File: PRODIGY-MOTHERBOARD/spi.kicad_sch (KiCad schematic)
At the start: 3 parts, among them U13 TXS0108EPW

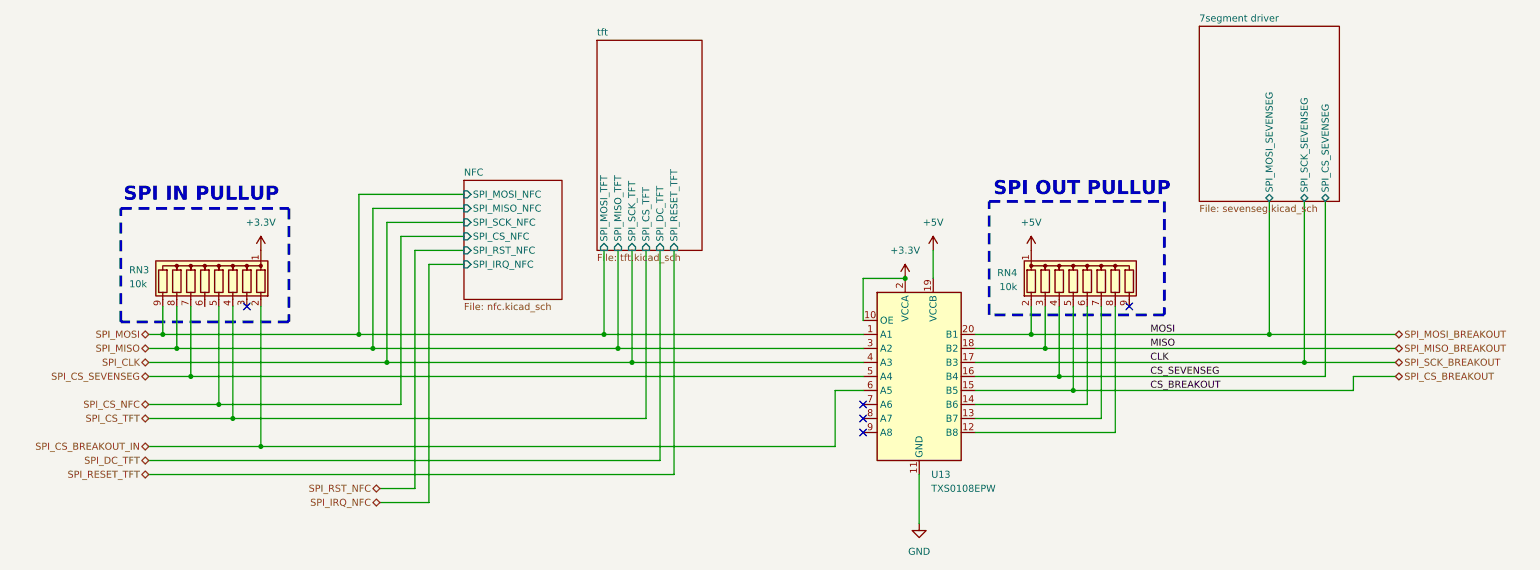
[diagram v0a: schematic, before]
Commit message: schematic v0.2 finalized
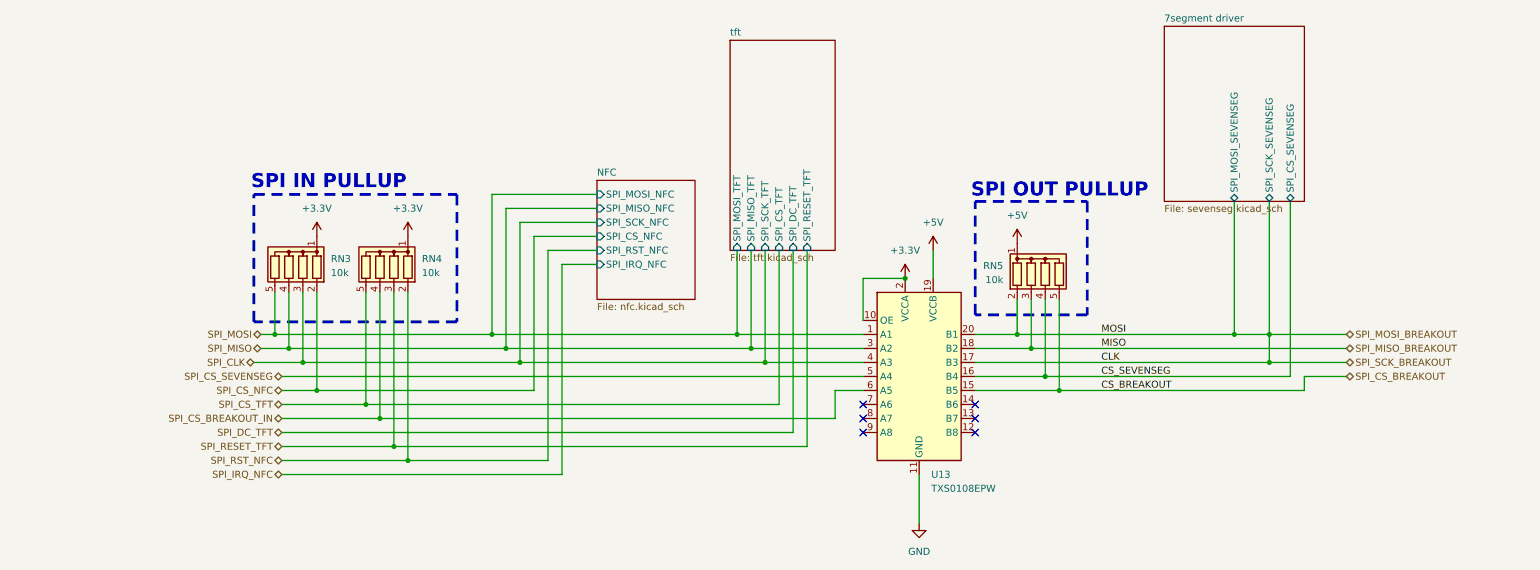
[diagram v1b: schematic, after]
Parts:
- removed RN3, RN4: 10k, Resistor_SMD:R_Array_Convex_5x0603, symbol Device:R_Network08
- added RN3, RN4, RN5: 10k, Resistor_SMD:R_Array_Convex_4x0603, symbol Device:R_Network04
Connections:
- net SPI_SCK_BREAKOUT is gone; now on net SPI_MOSI_BREAKOUT: U13.17 (B3)
- net +3.3V: now also RN3.1 (common), RN4.1 (common)
- net +5V: now also RN5.1 (common)
- net CS_SEVENSEG: now also RN5.4 (R3)
- net SPI_CLK: now also RN3.3 (R2)
- net SPI_CS_BREAKOUT: now also RN5.5 (R4)
- net SPI_CS_BREAKOUT_IN: now also RN4.4 (R3)
- net SPI_CS_NFC: now also RN3.2 (R1)
- net SPI_CS_TFT: now also RN4.5 (R4)
- net SPI_MISO: now also RN3.4 (R3)
- net SPI_MISO_BREAKOUT: now also RN5.3 (R2)
- net SPI_MOSI: now also RN3.5 (R4)
- net SPI_MOSI_BREAKOUT: now also RN5.2 (R1)
- net SPI_RESET_TFT: now also RN4.3 (R2)
- net SPI_RST_NFC: now also RN4.2 (R1)
- no-connect marks 5 -> 6
